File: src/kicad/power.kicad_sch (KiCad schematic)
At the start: 1 part, among them J2 USB_C_Receptacle_USB2.0_16P

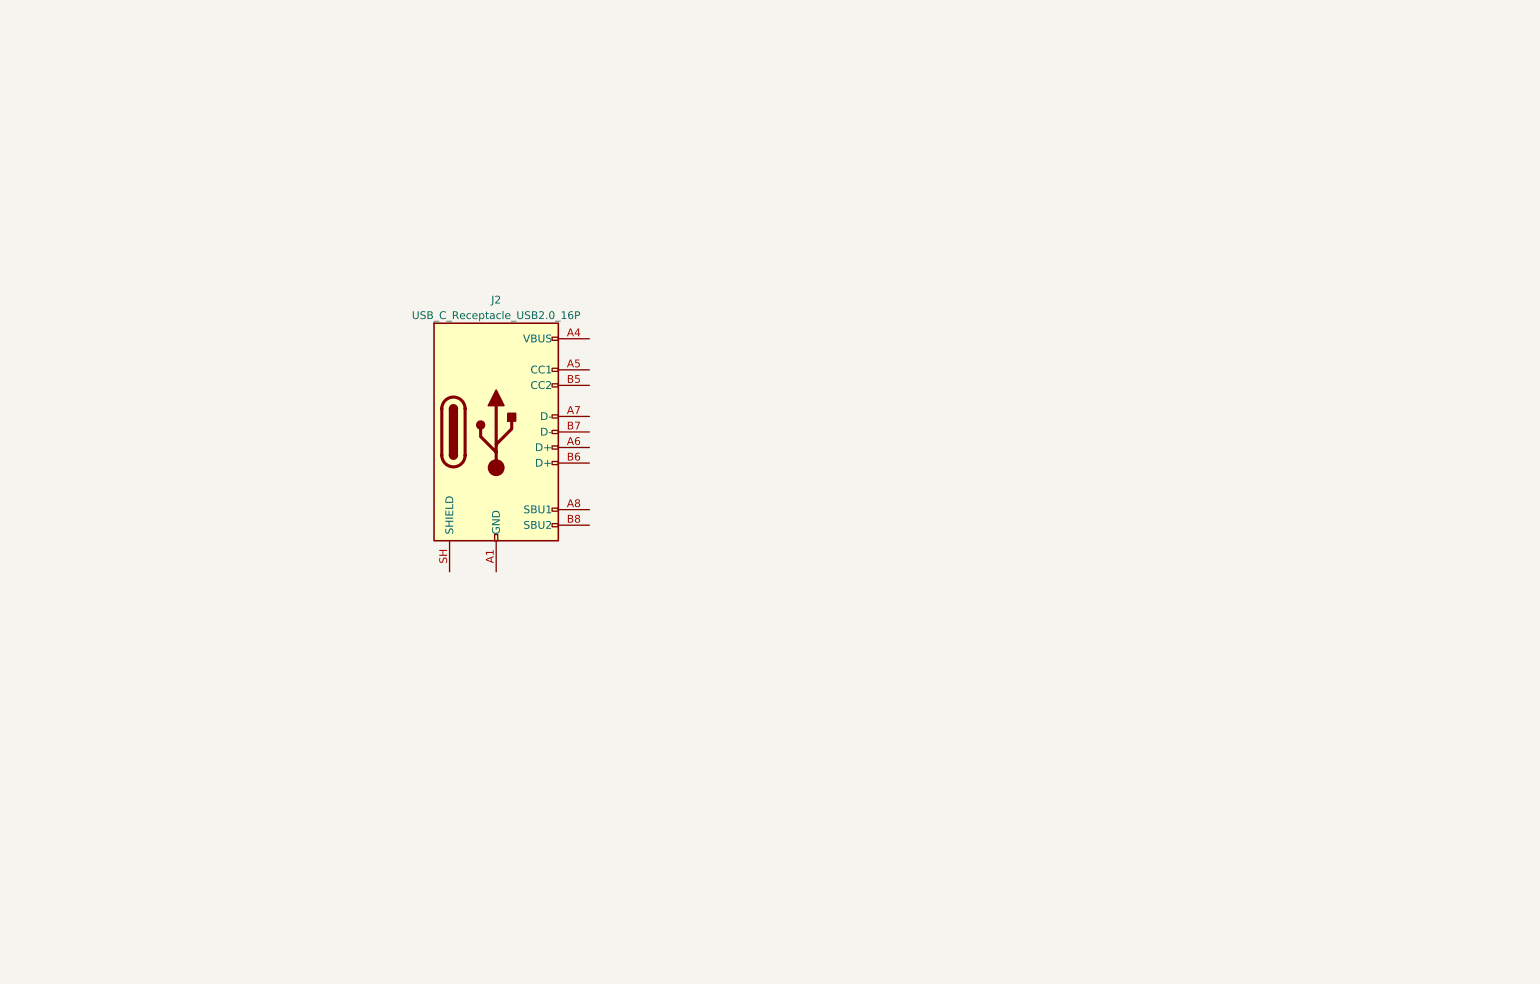
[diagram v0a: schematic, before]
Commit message: new day + schematic updates
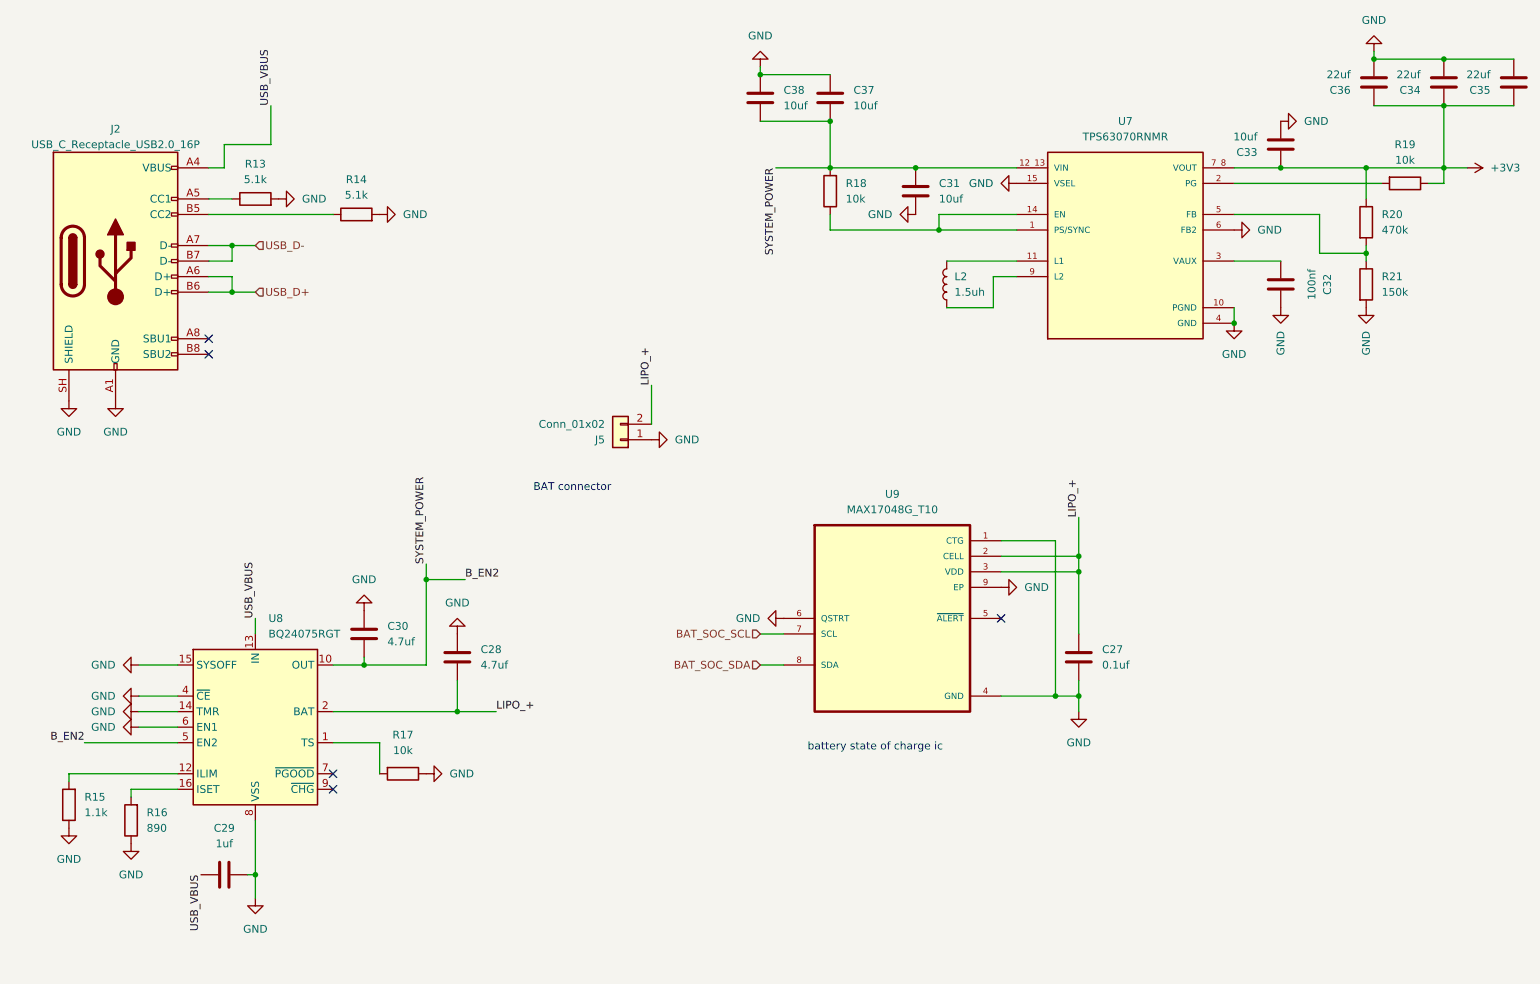
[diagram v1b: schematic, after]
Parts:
- added C27: 0.1uf, symbol Device:C
- added C28, C30: 4.7uf, symbol Device:C
- added C29: 1uf, symbol Device:C
- added C31, C33, C37, C38: 10uf, symbol Device:C
- added C32: 100nf, symbol Device:C
- added C34, C35, C36: 22uf, symbol Device:C
- added J5: Conn_01x02, symbol Connector_Generic:Conn_01x02
- added L2: 1.5uh, symbol Device:L
- added R13, R14: 5.1k, symbol Device:R
- added R15: 1.1k, symbol Device:R
- added R16: 890, symbol Device:R
- added R17, R18, R19: 10k, symbol Device:R
- added R20: 470k, symbol Device:R
- added R21: 150k, symbol Device:R
- added U7: TPS63070RNMR, TPS63070RNMR:VREG_TPS63070RNMR, symbol project_symbols:TPS63070RNMR
- added U8: BQ24075RGT, Package_DFN_QFN:VQFN-16-1EP_3x3mm_P0.5mm_EP1.6x1.6mm, symbol Battery_Management:BQ24075RGT
- added U9: MAX17048G_T10, max:SON50P200X200X80-9N, symbol project_symbols:MAX17048G_T10
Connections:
- net GND: now reaches J2.A1 (GND), J2.A12 (GND), J2.B1 (GND), J2.B12 (GND)
- net GND: now also J2.SH (SHIELD), C27.2, C28.1, C29.1, C30.1, C31.2, C32.2, C33.2, C34.2, C35.2, C36.2, C37.2, C38.1, J5.1 (Pin_1), R13.2, R14.2, R15.1, R16.1, R17.1, R21.2, U7.10 (PGND), U7.15 (VSEL), U7.4 (GND), U7.6 (FB2), U8.14 (TMR), U8.15 (SYSOFF), U8.17 (VSS), U8.4 (~{CE}), U8.6 (EN1), U8.8 (VSS), U9.1 (CTG), U9.4 (GND), U9.6 (QSTRT), U9.9 (EP)
- net USB_VBUS: now reaches J2.A4 (VBUS), J2.A9 (VBUS), J2.B4 (VBUS), J2.B9 (VBUS)
- net USB_VBUS: now also C29.2, U8.13 (IN)
- net at J2.A5 (CC1): now also R13.1
- net USB_D+: now reaches J2.A6 (D+)
- net USB_D+: now also J2.B6 (D+)
- net USB_D-: now reaches J2.A7 (D-)
- net USB_D-: now also J2.B7 (D-)
- net at J2.B5 (CC2): now also R14.1
- new net: C32.1, U7.3 (VAUX)
- new net: R15.2, U8.12 (ILIM)
- new net: R19.2, U7.2 (PG)
- new net: R18.1, U7.1 (PS/SYNC), U7.14 (EN)
- new net: L2.1, U7.9 (L2)
- new net: L2.2, U7.11 (L1)
- new net: R16.2, U8.16 (ISET)
- new net: R17.2, U8.1 (TS)
- new net: R20.2, R21.1, U7.5 (FB)
- new net +3V3: C33.1, C34.1, C35.1, C36.1, R19.1, R20.1, U7.7_8 (VOUT)
- new net BAT_SOC_SCL: U9.7 (SCL)
- new net BAT_SOC_SDA: U9.8 (SDA)
- new net B_EN2: C30.2, C31.1, C37.1, C38.2, R18.2, U7.12_13 (VIN), U8.10 (OUT), U8.11 (OUT), U8.5 (EN2)
- new net LIPO_+: C27.1, C28.2, J5.2 (Pin_2), U8.2 (BAT), U8.3 (BAT), U9.2 (CELL), U9.3 (VDD)
- no-connect marks 0 -> 5
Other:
- note added: "BAT connector"
- note added: "battery state of charge ic"
- moved on the sheet: J2

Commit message: new journal entry!
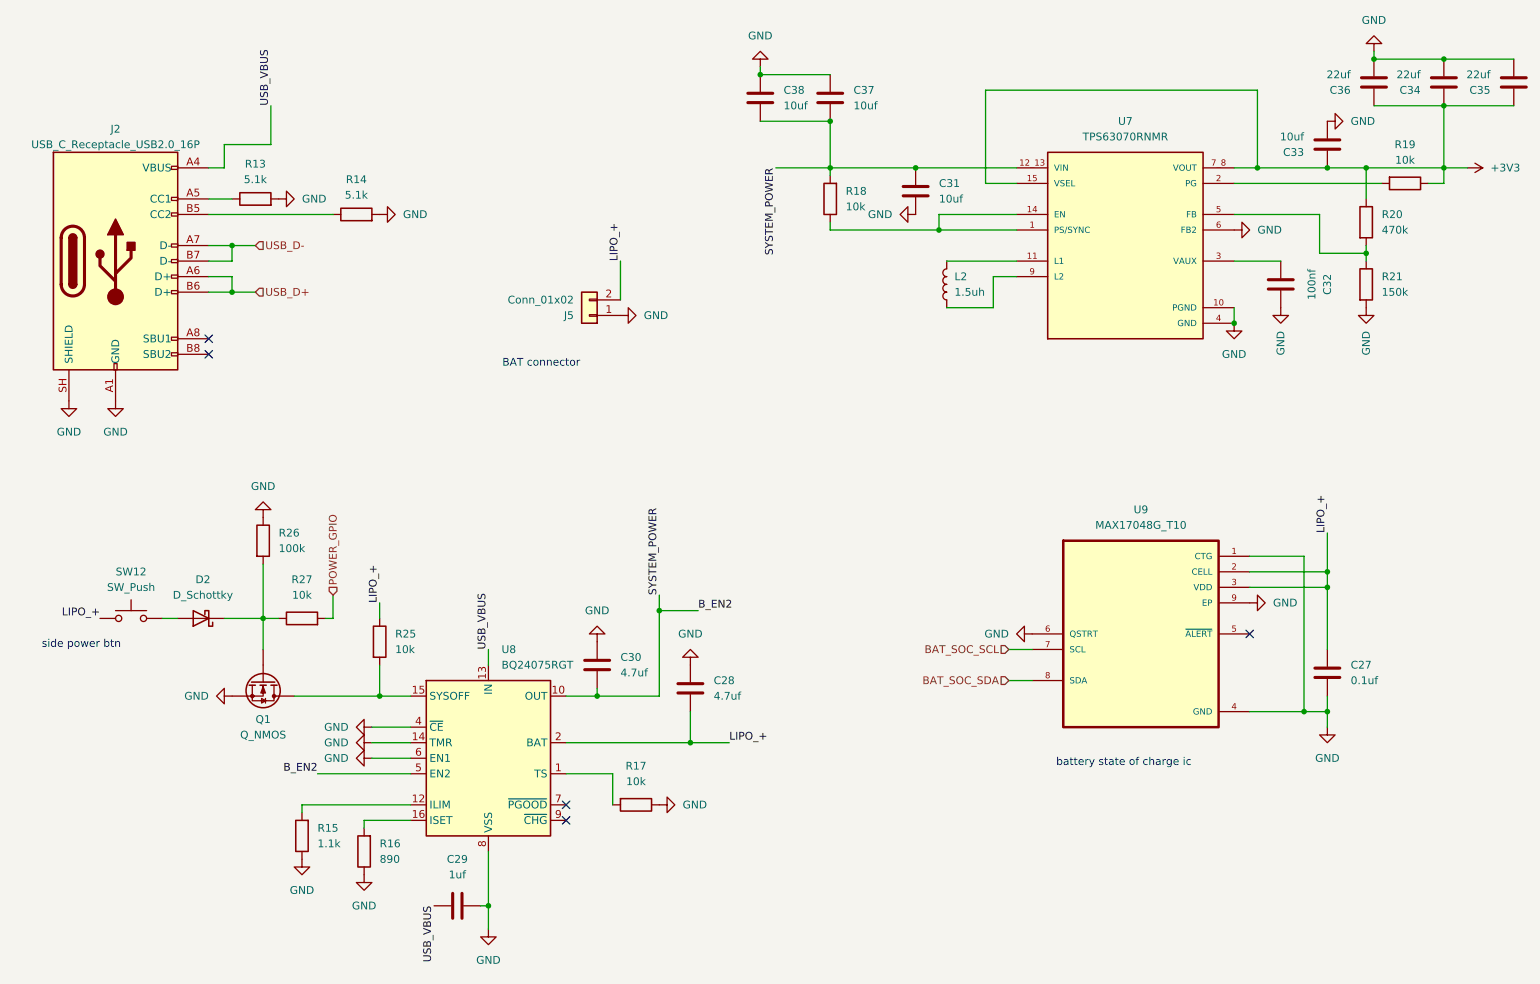
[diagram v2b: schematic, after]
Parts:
- added D2: D_Schottky, symbol Device:D_Schottky
- added Q1: Q_NMOS, symbol Device:Q_NMOS
- added R25, R27: 10k, symbol Device:R
- added R26: 100k, symbol Device:R
- added SW12: SW_Push, symbol Switch:SW_Push
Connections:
- net +3V3: now also U7.15 (VSEL)
- net GND: now also Q1.S, R26.1; no longer U7.15 (VSEL), U8.15 (SYSOFF)
- net LIPO_+: now also R25.1, SW12.1
- new net: Q1.D, R25.2, U8.15 (SYSOFF)
- new net: D2.2 (A), SW12.2
- new net: D2.1 (K), Q1.G, R26.2, R27.1
- new net POWER_GPIO: R27.2
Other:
- note added: "side power btn"
- moved on the sheet: C27, C28, C29, C30, C33, J5, R15, R16, R17, R18, U8, U9
